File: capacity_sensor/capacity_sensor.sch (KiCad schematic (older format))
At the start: 33 parts, among them J1 TP1, J2 Sensor, J3 TP2, J4 TP3, J5 Polarity, J6 TP4, J7 Pwr/Out, Q1 BC546, U1 ICM7555, U2 74HCT14, U3 74HC74

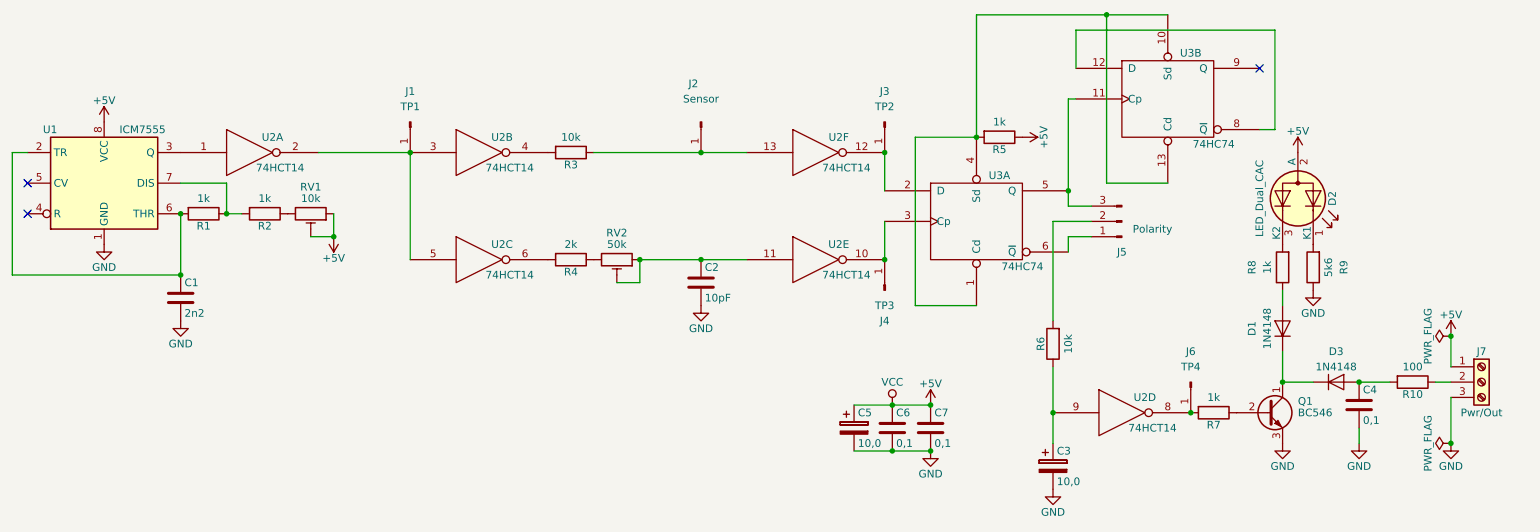
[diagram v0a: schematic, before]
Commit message: update
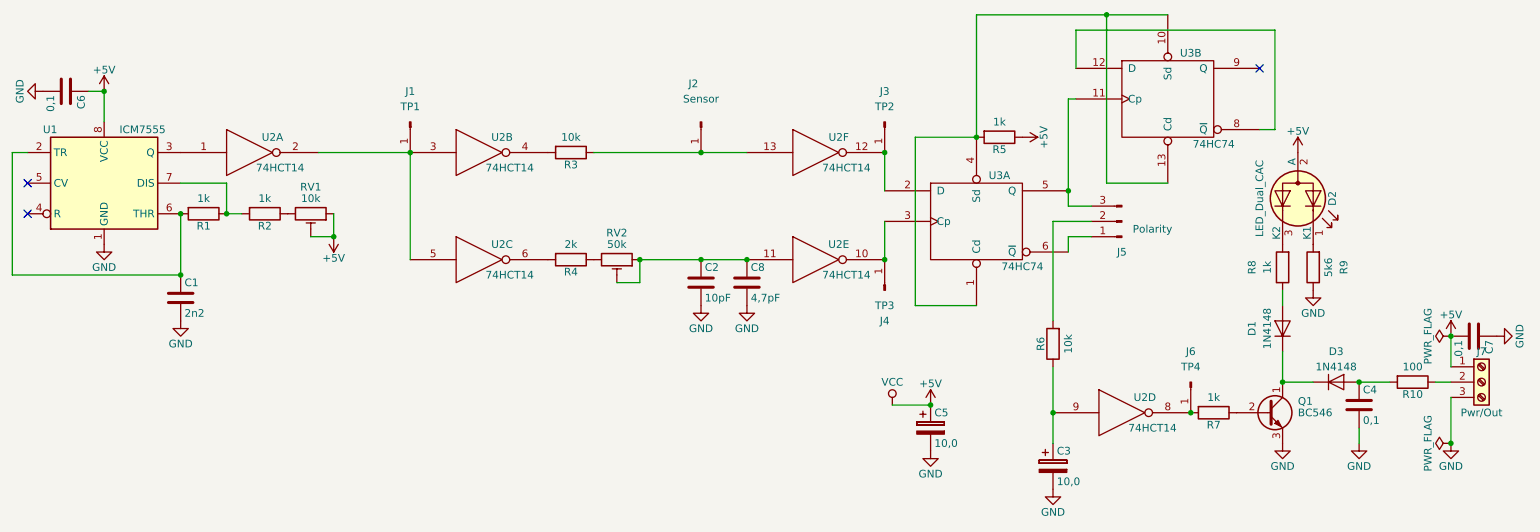
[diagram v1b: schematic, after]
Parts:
- added C8: 4,7pF, Capacitors_SMD:C_0805_HandSoldering, symbol C
- C6, C7: footprint (none) -> Capacitors_SMD:C_0805_HandSoldering
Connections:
- net +5V: now also C7.2; no longer C7.1
- net GND: now also C7.1, C8.2; no longer C7.2
- net at C2.1, RV2.1, RV2.2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: now also C8.1
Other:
- moved on the sheet: C5
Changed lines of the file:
@@
 LIBS:contrib
 LIBS:valves
+LIBS:capacity_sensor-cache
 EELAYER 25 0
 EELAYER END
@@
 $EndComp
 $Comp
-L +5V #PWR01
+L +5V #PWR2
 U 1 1 5A5778B9
-P 1800 1300
-F 0 "#PWR01" H 1800 1150 50  0001 C CNN
-F 1 "+5V" H 1800 1440 50  0000 C CNN
-F 2 "" H 1800 1300 50  0001 C CNN
-F 3 "" H 1800 1300 50  0001 C CNN
-	1    1800 1300
-	1    0    0    -1
-$EndComp
-$Comp
-L +5V #PWR02
+P 1800 1100
+F 0 "#PWR2" H 1800 950 50  0001 C CNN
+F 1 "+5V" H 1800 1240 50  0000 C CNN
+F 2 "" H 1800 1100 50  0001 C CNN
+F 3 "" H 1800 1100 50  0001 C CNN
+	1    1800 1100
+	1    0    0    -1
+$EndComp
+$Comp
+L +5V #PWR5
 U 1 1 5A5778E1
 P 3300 2050
-F 0 "#PWR02" H 3300 1900 50  0001 C CNN
+F 0 "#PWR5" H 3300 1900 50  0001 C CNN
 F 1 "+5V" H 3300 2190 50  0000 C CNN
 F 2 "" H 3300 2050 50  0001 C CNN
@@
 $EndComp
 $Comp
-L GND #PWR03
+L GND #PWR4
 U 1 1 5A5779DB
 P 2300 2600
-F 0 "#PWR03" H 2300 2350 50  0001 C CNN
+F 0 "#PWR4" H 2300 2350 50  0001 C CNN
 F 1 "GND" H 2300 2450 50  0000 C CNN
 F 2 "" H 2300 2600 50  0001 C CNN
@@
 $EndComp
 $Comp
-L GND #PWR04
+L GND #PWR3
 U 1 1 5A5779F9
 P 1800 2100
-F 0 "#PWR04" H 1800 1850 50  0001 C CNN
+F 0 "#PWR3" H 1800 1850 50  0001 C CNN
 F 1 "GND" H 1800 1950 50  0000 C CNN
 F 2 "" H 1800 2100 50  0001 C CNN
@@
 $EndComp
 $Comp
-L +5V #PWR05
+L +5V #PWR11
 U 1 1 5A5782D7
 P 7800 1400
-F 0 "#PWR05" H 7800 1250 50  0001 C CNN
+F 0 "#PWR11" H 7800 1250 50  0001 C CNN
 F 1 "+5V" H 7800 1540 50  0000 C CNN
 F 2 "" H 7800 1400 50  0001 C CNN
@@
 Connection ~ 5700 2200
 $Comp
-L GND #PWR06
+L GND #PWR6
 U 1 1 5A578985
 P 5700 2500
-F 0 "#PWR06" H 5700 2250 50  0001 C CNN
+F 0 "#PWR6" H 5700 2250 50  0001 C CNN
 F 1 "GND" H 5700 2350 50  0000 C CNN
 F 2 "" H 5700 2500 50  0001 C CNN
@@
 $EndComp
 $Comp
-L GND #PWR07
+L GND #PWR12
 U 1 1 5A578B94
 P 8000 3700
-F 0 "#PWR07" H 8000 3450 50  0001 C CNN
+F 0 "#PWR12" H 8000 3450 50  0001 C CNN
 F 1 "GND" H 8000 3550 50  0000 C CNN
 F 2 "" H 8000 3700 50  0001 C CNN
@@
 $EndComp
 $Comp
-L GND #PWR08
+L GND #PWR13
 U 1 1 5A5796EB
 P 9500 3400
-F 0 "#PWR08" H 9500 3150 50  0001 C CNN
+F 0 "#PWR13" H 9500 3150 50  0001 C CNN
 F 1 "GND" H 9500 3250 50  0000 C CNN
 F 2 "" H 9500 3400 50  0001 C CNN
@@
 $EndComp
 $Comp
-L GND #PWR09
+L GND #PWR16
 U 1 1 5A5798C3
 P 10000 3400
-F 0 "#PWR09" H 10000 3150 50  0001 C CNN
+F 0 "#PWR16" H 10000 3150 50  0001 C CNN
 F 1 "GND" H 10000 3250 50  0000 C CNN
 F 2 "" H 10000 3400 50  0001 C CNN
@@
 $EndComp
 $Comp
-L GND #PWR010
+L GND #PWR15
 U 1 1 5A579B51
 P 9700 2400
-F 0 "#PWR010" H 9700 2150 50  0001 C CNN
+F 0 "#PWR15" H 9700 2150 50  0001 C CNN
 F 1 "GND" H 9700 2250 50  0000 C CNN
 F 2 "" H 9700 2400 50  0001 C CNN
@@
 $EndComp
 $Comp
-L +5V #PWR011
+L +5V #PWR14
 U 1 1 5A579FA7
 P 9600 1500
-F 0 "#PWR011" H 9600 1350 50  0001 C CNN
+F 0 "#PWR14" H 9600 1350 50  0001 C CNN
 F 1 "+5V" H 9600 1640 50  0000 C CNN
 F 2 "" H 9600 1500 50  0001 C CNN
@@
 	10500 3000 10600 3000
 $Comp
-L GND #PWR012
+L GND #PWR18
 U 1 1 5A57A2D9
 P 10600 3400
-F 0 "#PWR012" H 10600 3150 50  0001 C CNN
+F 0 "#PWR18" H 10600 3150 50  0001 C CNN
 F 1 "GND" H 10600 3250 50  0000 C CNN
 F 2 "" H 10600 3400 50  0001 C CNN
@@
 	10600 3100 10600 3400
 $Comp
-L +5V #PWR013
+L +5V #PWR17
 U 1 1 5A57A38F
 P 10600 2700
-F 0 "#PWR013" H 10600 2550 50  0001 C CNN
+F 0 "#PWR17" H 10600 2550 50  0001 C CNN
 F 1 "+5V" H 10600 2840 50  0000 C CNN
 F 2 "" H 10600 2700 50  0001 C CNN
@@
 NoConn ~ 1300 1700
 $Comp
-L PWR_FLAG #FLG014
+L PWR_FLAG #FLG2
 U 1 1 5A57B75E
 P 10600 3400
-F 0 "#FLG014" H 10600 3475 50  0001 C CNN
+F 0 "#FLG2" H 10600 3475 50  0001 C CNN
 F 1 "PWR_FLAG" H 10600 3550 50  0000 C CNN
 F 2 "" H 10600 3400 50  0001 C CNN
@@
 $EndComp
 $Comp
-L PWR_FLAG #FLG015
+L PWR_FLAG #FLG1
 U 1 1 5A57B7D9
 P 10600 2700
-F 0 "#FLG015" H 10600 2775 50  0001 C CNN
+F 0 "#FLG1" H 10600 2775 50  0001 C CNN
 F 1 "PWR_FLAG" H 10600 2850 50  0000 C CNN
 F 2 "" H 10600 2700 50  0001 C CNN
@@
 Connection ~ 8000 3200
 $Comp
-L C C6
-U 1 1 5A57CFF5
-P 6950 3300
-F 0 "C6" H 6975 3400 50  0000 L CNN
-F 1 "0,1" H 6975 3200 50  0000 L CNN
-F 2 "" H 6988 3150 50  0001 C CNN
-F 3 "" H 6950 3300 50  0001 C CNN
-	1    6950 3300
-	1    0    0    -1
-$EndComp
-$Comp
-L C C7
-U 1 1 5A57D11D
+L CP C5
+U 1 1 5A57D1AC
 P 7200 3300
-F 0 "C7" H 7225 3400 50  0000 L CNN
-F 1 "0,1" H 7225 3200 50  0000 L CNN
-F 2 "" H 7238 3150 50  0001 C CNN
+F 0 "C5" H 7225 3400 50  0000 L CNN
+F 1 "10,0" H 7225 3200 50  0000 L CNN
+F 2 "Capacitors_Tantalum_SMD:CP_Tantalum_Case-B_EIA-3528-21_Hand" H 7238 3150 50  0001 C CNN
 F 3 "" H 7200 3300 50  0001 C CNN
 	1    7200 3300
@@
 $EndComp
 $Comp
-L CP C5
-U 1 1 5A57D1AC
-P 6700 3300
-F 0 "C5" H 6725 3400 50  0000 L CNN
-F 1 "10,0" H 6725 3200 50  0000 L CNN
-F 2 "Capacitors_Tantalum_SMD:CP_Tantalum_Case-B_EIA-3528-21_Hand" H 6738 3150 50  0001 C CNN
-F 3 "" H 6700 3300 50  0001 C CNN
-	1    6700 3300
-	1    0    0    -1
-$EndComp
-$Comp
-L GND #PWR016
+L GND #PWR10
 U 1 1 5A57D24E
 P 7200 3450
-F 0 "#PWR016" H 7200 3200 50  0001 C CNN
+F 0 "#PWR10" H 7200 3200 50  0001 C CNN
 F 1 "GND" H 7200 3300 50  0000 C CNN
 F 2 "" H 7200 3450 50  0001 C CNN
@@
 $EndComp
 $Comp
-L +5V #PWR017
+L +5V #PWR9
 U 1 1 5A57D2CB
 P 7200 3150
-F 0 "#PWR017" H 7200 3000 50  0001 C CNN
+F 0 "#PWR9" H 7200 3000 50  0001 C CNN
 F 1 "+5V" H 7200 3290 50  0000 C CNN
 F 2 "" H 7200 3150 50  0001 C CNN
@@
 	1    0    0    -1
 $EndComp
-Wire Wire Line
-	6700 3150 7200 3150
-Connection ~ 6950 3150
-Wire Wire Line
-	6700 3450 7200 3450
-Connection ~ 6950 3450
-Connection ~ 7200 3450
 Connection ~ 7200 3150
 $Comp
@@
 Connection ~ 8100 1750
 $Comp
-L VCC #PWR018
+L VCC #PWR8
 U 1 1 5A57D9BB
 P 6950 3150
-F 0 "#PWR018" H 6950 3000 50  0001 C CNN
+F 0 "#PWR8" H 6950 3000 50  0001 C CNN
 F 1 "VCC" H 6950 3300 50  0000 C CNN
 F 2 "" H 6950 3150 50  0001 C CNN
@@
 $EndComp
 NoConn ~ 9350 950
+Wire Wire Line
+	1700 1100 1800 1100
+Wire Wire Line
+	1800 1100 1800 1300
+Connection ~ 1800 1100
+$Comp
+L GND #PWR1
+U 1 1 5A57BA2A
+P 1400 1100
+F 0 "#PWR1" H 1400 850 50  0001 C CNN
+F 1 "GND" H 1400 950 50  0000 C CNN
+F 2 "" H 1400 1100 50  0001 C CNN
+F 3 "" H 1400 1100 50  0001 C CNN
+	1    1400 1100
+	0    1    1    0
+$EndComp
+$Comp
+L GND #PWR19
+U 1 1 5A57BEB3
+P 10900 2700
+F 0 "#PWR19" H 10900 2450 50  0001 C CNN
+F 1 "GND" H 10900 2550 50  0000 C CNN
+F 2 "" H 10900 2700 50  0001 C CNN
+F 3 "" H 10900 2700 50  0001 C CNN
+	1    10900 2700
+	0    -1   -1   0
+$EndComp
+Wire Wire Line
+	6950 3150 7200 3150
+$Comp
+L C C6
+U 1 1 5A57C71D
+P 1550 1100
+F 0 "C6" H 1575 1200 50  0000 L CNN
+F 1 "0,1" H 1575 1000 50  0000 L CNN
+F 2 "Capacitors_SMD:C_0805_HandSoldering" H 1588 950 50  0001 C CNN
+F 3 "" H 1550 1100 50  0000 C CNN
+	1    1550 1100
+	0    1    1    0
+$EndComp
+$Comp
+L C C7
+U 1 1 5A57CB5F
+P 10750 2700
+F 0 "C7" H 10775 2800 50  0000 L CNN
+F 1 "0,1" H 10775 2600 50  0000 L CNN
+F 2 "Capacitors_SMD:C_0805_HandSoldering" H 10788 2550 50  0001 C CNN
+F 3 "" H 10750 2700 50  0000 C CNN
+	1    10750 2700
+	0    1    1    0
+$EndComp
+$Comp
+L C C8
+U 1 1 5A5F5345
+P 6000 2350
+F 0 "C8" H 6025 2450 50  0000 L CNN
+F 1 "4,7pF" H 6025 2250 50  0000 L CNN
+F 2 "Capacitors_SMD:C_0805_HandSoldering" H 6038 2200 50  0001 C CNN
+F 3 "" H 6000 2350 50  0001 C CNN
+	1    6000 2350
+	1    0    0    -1
+$EndComp
+$Comp
+L GND #PWR7
+U 1 1 5A5F53D1
+P 6000 2500
+F 0 "#PWR7" H 6000 2250 50  0001 C CNN
+F 1 "GND" H 6000 2350 50  0000 C CNN
+F 2 "" H 6000 2500 50  0001 C CNN
+F 3 "" H 6000 2500 50  0001 C CNN
+	1    6000 2500
+	1    0    0    -1
+$EndComp
+Connection ~ 6000 2200
 $EndSCHEMATC
